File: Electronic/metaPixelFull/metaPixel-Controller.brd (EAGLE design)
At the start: 81.3 x 64.8 mm, 17 parts, among them IC1 MAX481CPA, IC2 TEENSY_3.1, IC3 74HCT245N

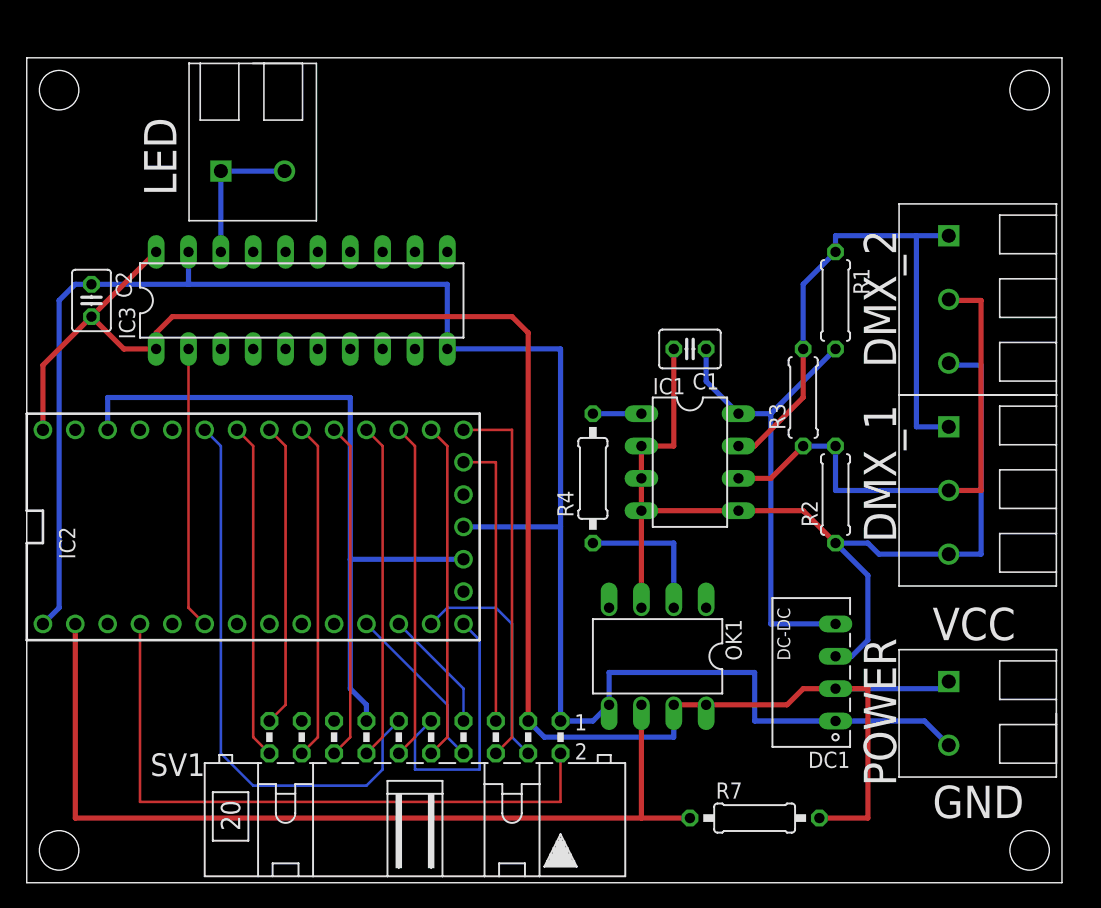
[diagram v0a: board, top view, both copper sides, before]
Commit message: Fixing the boards
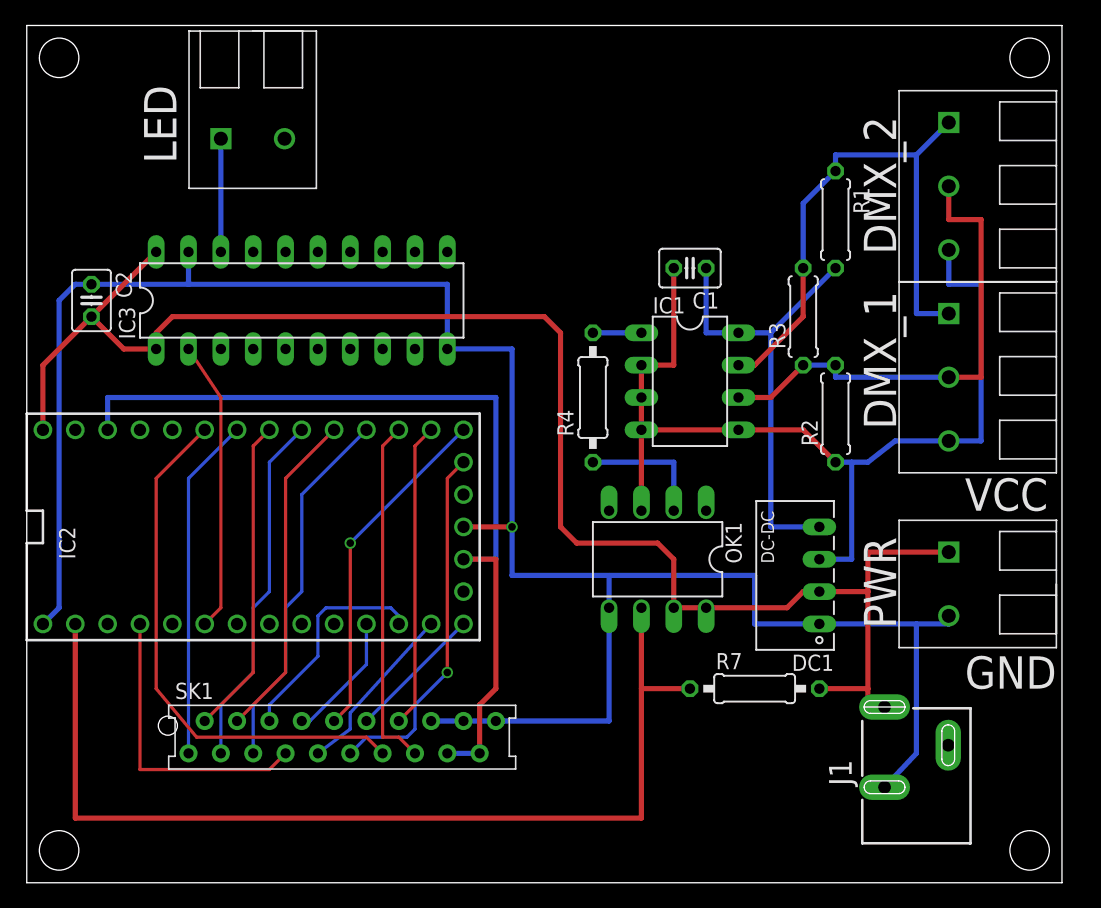
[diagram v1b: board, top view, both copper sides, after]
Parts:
- removed POWER: RP025-02, RP025xx:RP025-02
- removed SV1: DISPLAY, con-harting-ml:ML20L
- added J1: PWR, SparkFun-Connectors:POWER_JACK_SLOT
- added PWR: RP025-02, RP025xx:RP025-02
- added SK1: Display, jt-con-micromatch:AMP-215079-20
- moved R7 10.2 mm to (57.1, 15.2)
- moved DMX_1 8.89 mm to (72.4, 44.7)
- moved DMX_2 8.89 mm to (72.4, 59.7)
- moved DC1 7.73 mm to (62.2, 24.1)
- moved OK1 7.62 mm to (49.5, 25.4)
- moved C1 6.35 mm to (52.1, 48.3)
- moved R1 6.35 mm to (63.5, 52.1)
- moved R3 6.35 mm to (61.0, 44.5)
- moved R4 6.35 mm to (44.5, 38.1)
- moved R2 6.35 mm to (63.5, 36.8)
- moved IC1 6.35 mm to (52.1, 39.4)
- moved LED 2.54 mm to (15.2, 58.4)
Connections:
- removed net !SD_CS: IC2.21/A7, SV1.11
- removed net ENC_DIR: IC2.20/A6, SV1.20
- removed net ENC_STEP: IC2.19/A5, SV1.19
- new net !MEM_CS: IC2.21/A7, SK1.13
- new net ENC_A: IC2.14/A0, SK1.14
- new net ENC_B: IC2.15/A1, SK1.15
- net !LCD_CS: now also SK1.6; no longer SV1.7
- net !LCD_RST: now also SK1.7; no longer SV1.2
- net +3.3V: now also SK1.17, SK1.19; no longer SV1.13
- net GND: now also J1.GND@1, PWR.P$2, SK1.16, SK1.18, SK1.20; no longer POWER.P$2, SV1.1
- net KEY_1: now also IC2.20/A6, SK1.1; no longer IC2.14/A0, SV1.10
- net KEY_2: now also IC2.19/A5, SK1.2; no longer IC2.15/A1, SV1.12
- net KEY_3: now also IC2.18/A4, SK1.3; no longer IC2.16/A2, SV1.14
- net KEY_4: now also SK1.4; no longer SV1.16
- net KEY_5: now also IC2.16/A2, SK1.5; no longer IC2.18/A4, SV1.18
- net LCD_DC: now also SK1.8; no longer SV1.8
- net LCD_LED: now also SK1.11; no longer SV1.5
- net LED_OUT: no longer LED.P$2
- net MISO: now also SK1.12; no longer SV1.9
- net MOSI: now also SK1.9; no longer SV1.4
- net SCLK: now also SK1.10; no longer SV1.6
- net VCC: now also J1.PWR, PWR.P$1; no longer POWER.P$1, SV1.3
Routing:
- net !SD_CS: track 44.5 -> 0.00 mm
- net !MEM_CS: track 0.00 -> 42.0 mm
- net ENC_B: track 0.00 -> 27.7 mm
- net !LCD_RST: track 50.8 -> 23.4 mm
- net ENC_DIR: track 26.5 -> 0.00 mm
- net ENC_STEP: track 23.9 -> 0.00 mm
- net ENC_A: track 0.00 -> 23.9 mm
- net GND: track 148.4 -> 169.2 mm, vias 0 -> 1
- net VCC: track 139.2 -> 126.1 mm
- net +3.3V: track 56.4 -> 69.1 mm
- net MISO: track 21.4 -> 10.8 mm
- net !LCD_CS: track 9.72 -> 17.3 mm
- net DMX_IN: track 72.4 -> 80.0 mm
- net LCD_LED: track 22.9 -> 28.4 mm, vias 0 -> 1
- net MOSI: track 18.1 -> 13.9 mm
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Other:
- board size 81.3 x 64.8 mm -> 81.3 x 67.3 mm
